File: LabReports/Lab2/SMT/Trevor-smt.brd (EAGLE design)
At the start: 28.9 x 22.9 mm, 5 parts, among them J1 2.1MMJACKTHM

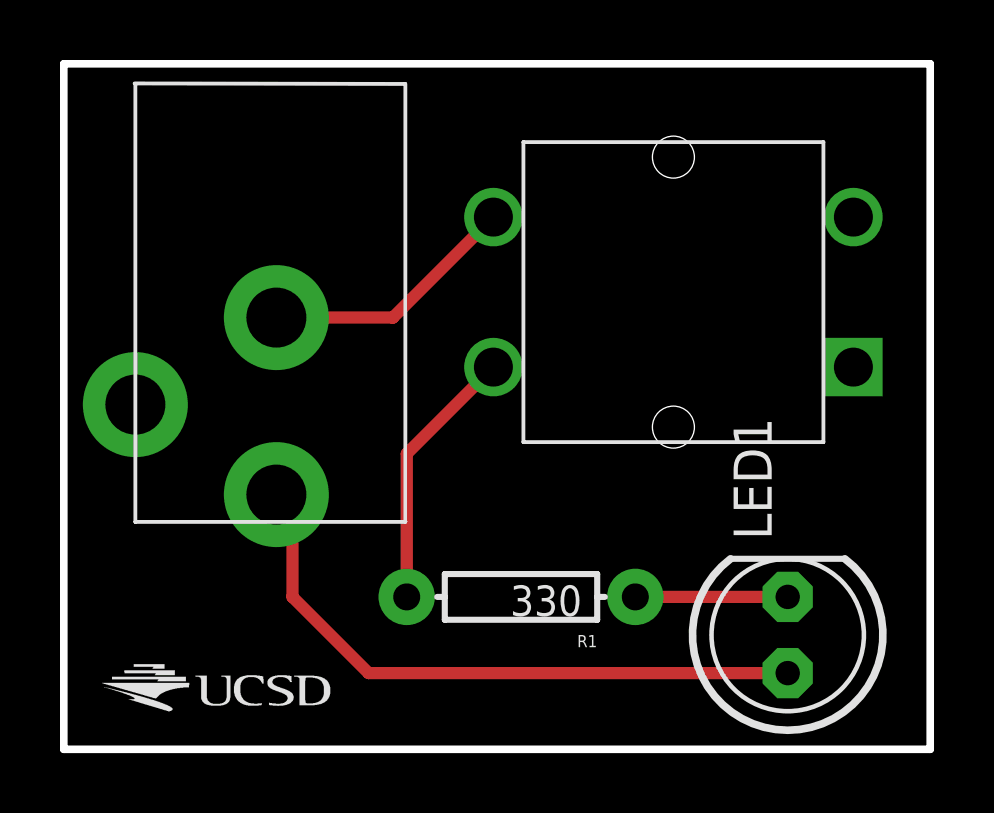
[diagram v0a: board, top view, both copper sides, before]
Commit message: Added SMT schematic and board
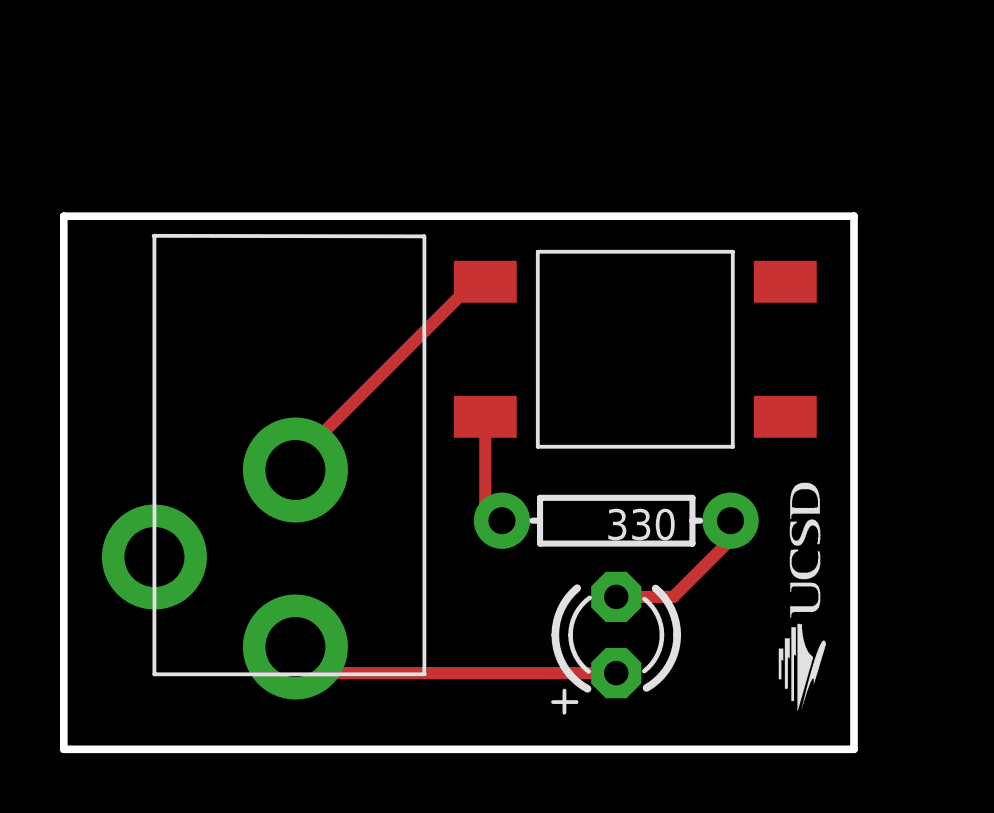
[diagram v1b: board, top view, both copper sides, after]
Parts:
- J1: device Lab2:PJ-102A -> Trevor-Lab2:PJ-102A
- LED1: value Red -> (none); device Lab2:LED5MM -> Trevor-Lab2:LED3MM
- R1: device Lab2:AXIAL-0.3 -> Trevor-Lab2:AXIAL-0.3
- S1: value BUTTON-TACTILE-SQUARE -> BUTTON-TACTILE-LSH; device Lab2:BUTTON-TACTILE-SQUARE-ADAFRUIT1010 -> Trevor-Lab2:1301.9315
- moved U$1 24.1 mm to (25.4, 1.27), turned to 90 degrees
- moved LED1 5.71 mm to (18.4, 3.81)
- moved J1 5.12 mm to (12.1, 2.54)
- moved R1 4.07 mm to (18.4, 7.62)
- moved S1 2.29 mm to (19.1, 13.3)
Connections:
- net N$3: now also S1.P$2; no longer S1.P2
- net N$4: now also S1.P$4; no longer S1.S2
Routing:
- net N$1: track 21.2 -> 11.1 mm
- net N$3: track 8.86 -> 3.69 mm
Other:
- board size 28.9 x 22.9 mm -> 26.3 x 17.8 mm
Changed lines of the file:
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@@
 <drawing>
 <settings>
-<setting alwaysvectorfont="no"/>
+<setting alwaysvectorfont="yes"/>
 <setting verticaltext="up"/>
 </settings>
-<grid distance="0.05" unitdist="inch" unit="inch" style="lines" multiple="1" display="no" altdistance="0.025" altunitdist="inch" altunit="inch"/>
+<grid distance="0.05" unitdist="inch" unit="inch" style="dots" multiple="1" display="yes" altdistance="0.025" altunitdist="inch" altunit="inch"/>
 <layers>
 <layer number="1" name="Top" color="4" fill="1" visible="yes" active="yes"/>
@@
 <board>
 <plain>
-<wire x1="0" y1="0" x2="28.88" y2="0" width="0.254" layer="20"/>
-<wire x1="28.88" y1="0" x2="28.88" y2="22.85" width="0.254" layer="20"/>
-<wire x1="28.88" y1="22.85" x2="0" y2="22.85" width="0.254" layer="20"/>
-<wire x1="0" y1="22.85" x2="0" y2="0" width="0.254" layer="20"/>
+<wire x1="0" y1="0" x2="26.34" y2="0" width="0.254" layer="20"/>
+<wire x1="26.34" y1="0" x2="26.34" y2="17.77" width="0.254" layer="20"/>
+<wire x1="26.34" y1="17.77" x2="0" y2="17.77" width="0.254" layer="20"/>
+<wire x1="0" y1="17.77" x2="0" y2="0" width="0.254" layer="20"/>
 </plain>
 <attributes>
@@
 </class>
 </classes>
-<designrules name="4pcb-33board">
+<designrules name="default">
 <description language="de">&lt;b&gt;EAGLE Design Rules&lt;/b&gt;
 &lt;p&gt;
@@
 design rules under a new name.</description>
 <param name="layerSetup" value="(1*16)"/>
-<param name="mtCopper" value="0.035559375mm 0.035559375mm 0.035559375mm 0.035559375mm 0.035559375mm 0.035559375mm 0.035559375mm 0.035559375mm 0.035559375mm 0.035559375mm 0.035559375mm 0.035559375mm 0.035559375mm 0.035559375mm 0.035559375mm 0.035559375mm"/>
-<param name="mtIsolate" value="1.501140625mm 0.149859375mm 0.200659375mm 0.149859375mm 0.200659375mm 0.149859375mm 0.200659375mm 0.149859375mm 0.200659375mm 0.149859375mm 0.200659375mm 0.149859375mm 0.200659375mm 0.149859375mm 0.200659375mm"/>
-<param name="mdWireWire" value="6mil"/>
-<param name="mdWirePad" value="6mil"/>
-<param name="mdWireVia" value="6mil"/>
-<param name="mdPadPad" value="6mil"/>
-<param name="mdPadVia" value="6mil"/>
-<param name="mdViaVia" value="6mil"/>
-<param name="mdSmdPad" value="6mil"/>
-<param name="mdSmdVia" value="6mil"/>
-<param name="mdSmdSmd" value="6mil"/>
+<param name="mtCopper" value="0.035mm 0.035mm 0.035mm 0.035mm 0.035mm 0.035mm 0.035mm 0.035mm 0.035mm 0.035mm 0.035mm 0.035mm 0.035mm 0.035mm 0.035mm 0.035mm"/>
+<param name="mtIsolate" value="1.5mm 0.15mm 0.2mm 0.15mm 0.2mm 0.15mm 0.2mm 0.15mm 0.2mm 0.15mm 0.2mm 0.15mm 0.2mm 0.15mm 0.2mm"/>
+<param name="mdWireWire" value="8mil"/>
+<param name="mdWirePad" value="8mil"/>
+<param name="mdWireVia" value="8mil"/>
+<param name="mdPadPad" value="8mil"/>
+<param name="mdPadVia" value="8mil"/>
+<param name="mdViaVia" value="8mil"/>
+<param name="mdSmdPad" value="8mil"/>
+<param name="mdSmdVia" value="8mil"/>
+<param name="mdSmdSmd" value="8mil"/>
 <param name="mdViaViaSameLayer" value="8mil"/>
 <param name="mnLayersViaInSmd" value="2"/>
-<param name="mdCopperDimension" value="10mil"/>
-<param name="mdDrill" value="10mil"/>
+<param name="mdCopperDimension" value="40mil"/>
+<param name="mdDrill" value="8mil"/>
 <param name="mdSmdStop" value="0mil"/>
 <param name="msWidth" value="10mil"/>
-<param name="msDrill" value="15mil"/>
-<param name="msMicroVia" value="9.98981875mm"/>
+<param name="msDrill" value="24mil"/>
+<param name="msMicroVia" value="9.99mm"/>
 <param name="msBlindViaRatio" value="0.5"/>
 <param name="rvPadTop" value="0.25"/>
@@
 </autorouter>
 <elements>
-<element name="J1" library="Lab2" package="PJ-102A" value="2.1MMJACKTHM" x="11.43" y="7.62" rot="R270"/>
-<element name="LED1" library="Lab2" package="LED5MM" value="Red" x="24.13" y="3.81" rot="R90"/>
-<element name="R1" library="Lab2" package="AXIAL-0.3" value="330" x="15.24" y="5.08" rot="R180"/>
-<element name="S1" library="Lab2" package="BUTTON-TACTILE-SQUARE-ADAFRUIT1010" value="BUTTON-TACTILE-SQUARE" x="20.32" y="15.24" rot="R180"/>
-<element name="U$1" library="Logo" package="UCSD_LOGO" value="" x="1.27" y="1.27"/>
+<element name="J1" library="Trevor-Lab2" package="PJ-102A" value="2.1MMJACKTHM" x="12.065" y="2.54" rot="R270"/>
+<element name="LED1" library="Trevor-Lab2" package="LED3MM" value="" x="18.415" y="3.81" smashed="yes" rot="R90">
+<attribute name="VALUE" x="20.066" y="5.715" size="1.27" layer="27" ratio="10" rot="R90"/>
+</element>
+<element name="R1" library="Trevor-Lab2" package="AXIAL-0.3" value="330" x="18.415" y="7.62" smashed="yes" rot="R180">
+<attribute name="VALUE" x="20.447" y="8.001" size="1.016" layer="21" font="vector" ratio="15" rot="R180"/>
+</element>
+<element name="S1" library="Trevor-Lab2" package="1301.9315" value="BUTTON-TACTILE-LSH" x="19.05" y="13.335" smashed="yes" rot="R180"/>
+<element name="U$1" library="Logo" package="UCSD_LOGO" value="" x="25.4" y="1.27" rot="R90"/>
 </elements>
 <signals>
@@
 <contactref element="J1" pad="TIP"/>
 <contactref element="LED1" pad="A"/>
-<wire x1="24.13" y1="2.54" x2="10.16" y2="2.54" width="0.4064" layer="1"/>
-<wire x1="10.16" y1="2.54" x2="7.62" y2="5.08" width="0.4064" layer="1"/>
-<wire x1="7.62" y1="5.08" x2="7.62" y2="7.955" width="0.4064" layer="1"/>
-<wire x1="7.62" y1="7.955" x2="7.085" y2="8.49" width="0.4064" layer="1"/>
+<wire x1="18.415" y1="2.54" x2="8.59" y2="2.54" width="0.4064" layer="1"/>
+<wire x1="8.59" y1="2.54" x2="7.72" y2="3.41" width="0.4064" layer="1"/>
 </signal>
 <signal name="N$2">
 <contactref element="LED1" pad="K"/>
 <contactref element="R1" pad="P$1"/>
-<wire x1="24.13" y1="5.08" x2="19.05" y2="5.08" width="0.4064" layer="1"/>
+<wire x1="22.225" y1="7.62" x2="22.225" y2="6.985" width="0.4064" layer="1"/>
+<wire x1="22.225" y1="6.985" x2="20.32" y2="5.08" width="0.4064" layer="1"/>
+<wire x1="20.32" y1="5.08" x2="18.415" y2="5.08" width="0.4064" layer="1"/>
 </signal>
 <signal name="N$3">
 <contactref element="R1" pad="P$2"/>
-<contactref element="S1" pad="P2"/>
-<wire x1="11.43" y1="5.08" x2="11.43" y2="9.85" width="0.4064" layer="1"/>
-<wire x1="11.43" y1="9.85" x2="14.32" y2="12.74" width="0.4064" layer="1"/>
+<contactref element="S1" pad="P$2"/>
+<wire x1="14.05" y1="11.085" x2="14.05" y2="8.175" width="0.4064" layer="1"/>
+<wire x1="14.05" y1="8.175" x2="14.605" y2="7.62" width="0.4064" layer="1"/>
 </signal>
 <signal name="N$4">
+<contactref element="S1" pad="P$4"/>
 <contactref element="J1" pad="RING"/>
-<contactref element="S1" pad="S2"/>
-<wire x1="7.085" y1="14.39" x2="10.97" y2="14.39" width="0.4064" layer="1"/>
-<wire x1="10.97" y1="14.39" x2="14.32" y2="17.74" width="0.4064" layer="1"/>
+<wire x1="7.72" y1="9.31" x2="7.72" y2="9.625" width="0.4064" layer="1"/>
+<wire x1="7.72" y1="9.625" x2="13.335" y2="15.24" width="0.4064" layer="1"/>
+<wire x1="13.335" y1="15.24" x2="13.705" y2="15.24" width="0.4064" layer="1"/>
+<wire x1="13.705" y1="15.24" x2="14.05" y2="15.585" width="0.4064" layer="1"/>
 </signal>
 </signals>
